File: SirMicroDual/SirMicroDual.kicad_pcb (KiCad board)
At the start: 2 copper layers, 50.8 x 20.5 mm, 48 parts, among them J1 Conn_01x16, J2 Conn_01x16, J3 USB_B_Micro, Q1 Q_DUAL_PMOS_S1G1D2S2G2D1, U1 ATmega32U4-MU, U2 AP2127K-3.3, U3 AP1117-50

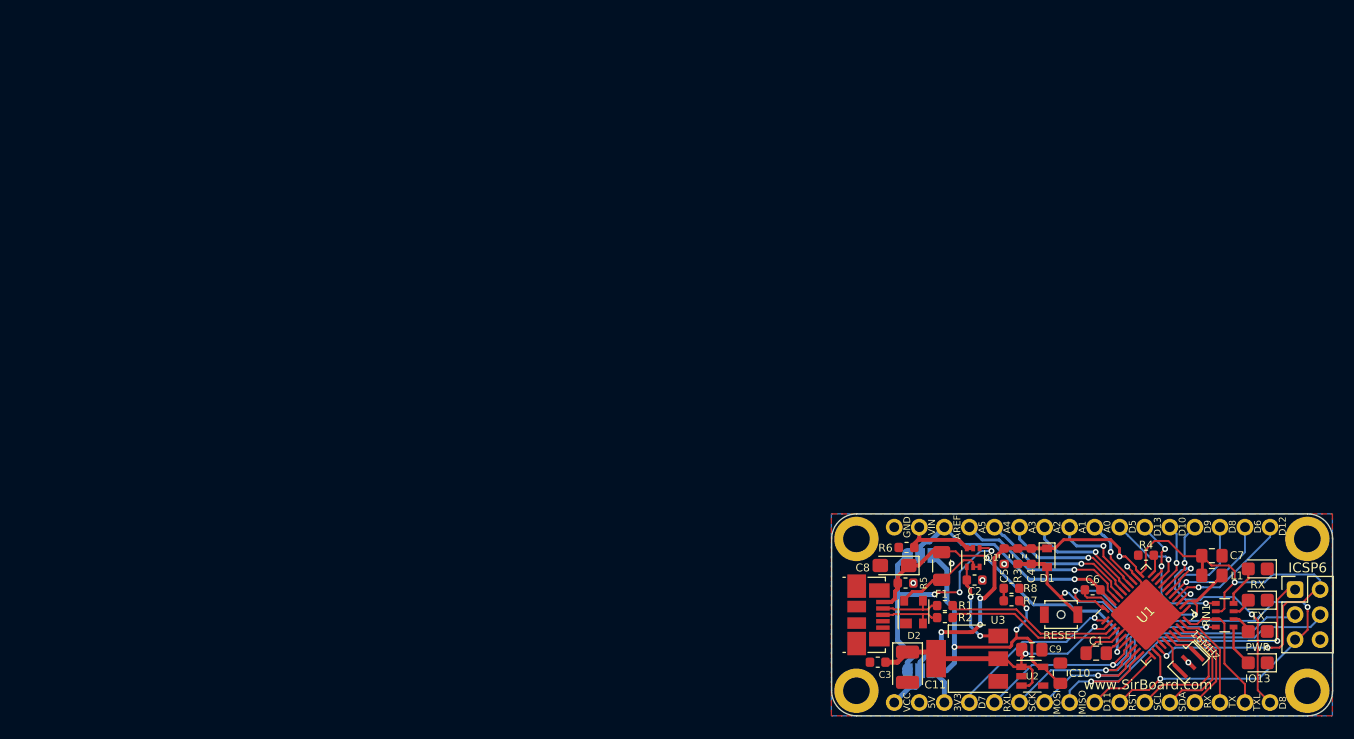
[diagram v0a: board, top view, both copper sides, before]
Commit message: Part Numbers Added
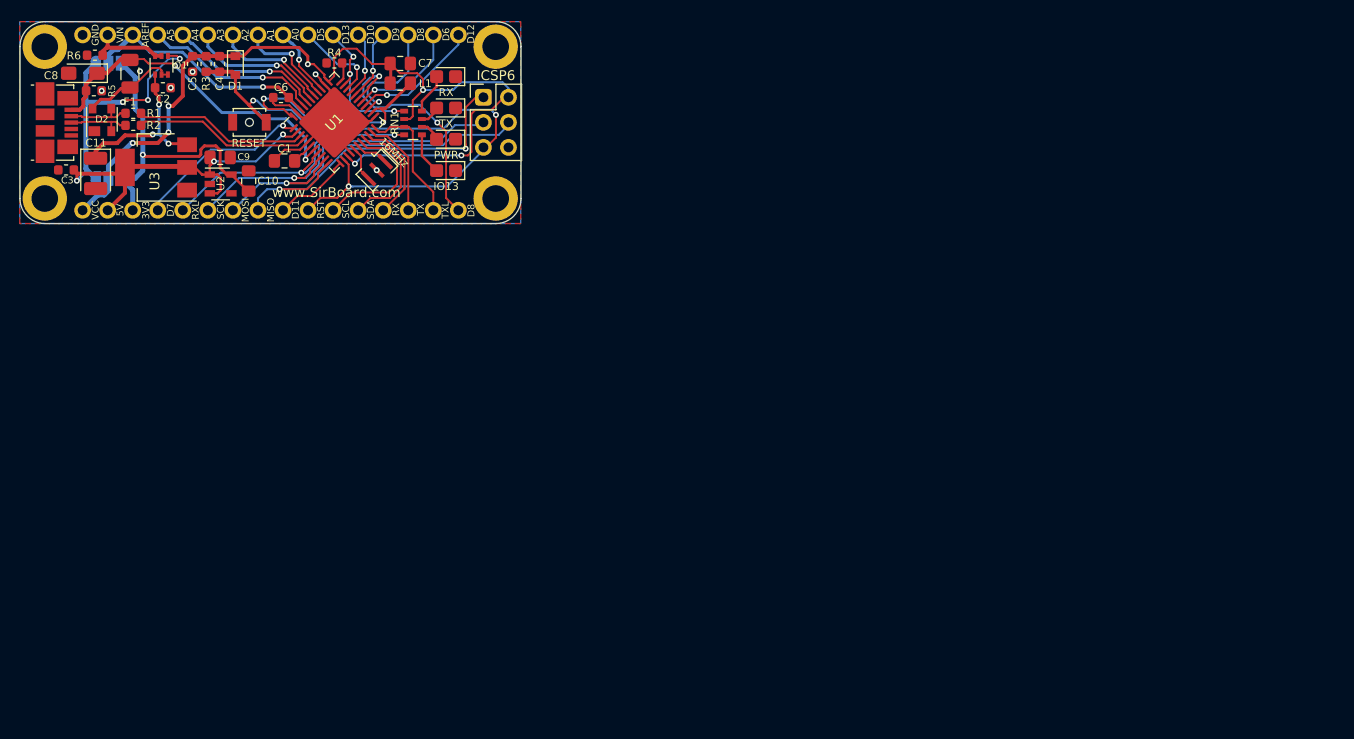
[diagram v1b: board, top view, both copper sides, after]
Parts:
- removed R7: 68K, Resistor_SMD:R_0603_1608Metric
- removed R8: 22K, Resistor_SMD:R_0603_1608Metric
- JP1, JP2: value SolderJumper_3_Bridged12 -> SolderJumper_3_Open
- Q1: value Q_DUAL_PMOS_S1G1D2S2G2D1 -> DMP2004DWK-7
- U3: value AP1117-50 -> AZ1117-5.0
- moved C11 96.3 mm to (51.3, 46.7)
- moved REF** 96.2 mm to (46.1, 49.3)
- moved REF** 96.2 mm to (46.1, 33.9)
- moved 16MHz 96.2 mm to (79.8, 46.4)
- moved C10 96.2 mm to (66.8, 47.5)
- moved C2 96.2 mm to (58.1, 38.0)
- moved C3 96.2 mm to (48.3, 46.4)
- moved C7 96.2 mm to (82.2, 35.6)
- moved C9 96.2 mm to (63.9, 45.1)
- moved D1 96.2 mm to (65.5, 35.8)
- moved D2 96.2 mm to (51.9, 41.2)
- moved F1 96.2 mm to (54.8, 36.6)
- moved G*** 96.2 mm to (51.2, 41.3)
- moved IO13 96.2 mm to (86.8, 46.4)
- moved J1 96.2 mm to (50.0, 32.7)
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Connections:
- C11 pad 1: 5V -> Net-(C11-Pad1)
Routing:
- net Net-(C11-Pad1): track 9.40 -> 17.3 mm, vias 2 -> 3
- net 5V: track 57.4 -> 65.1 mm, vias 5 -> 6
- net 3V3: track 36.8 -> 32.6 mm, vias 3 -> 1
- net Net-(R7-Pad2): track 1.27 -> 0.00 mm
